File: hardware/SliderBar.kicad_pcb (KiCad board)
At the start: 2 copper layers, 50 x 30.1 mm, 35 parts, among them J1 USB_B_Mini, J2 MOTOR, J3 TAPER_RIGHT, J4 TAPER_LEFT, J5 DEBUG, U1 MIC5205-3.3YM5, U2 MT3608, U3 STM32F072C8Tx, U4 TB6612FNG

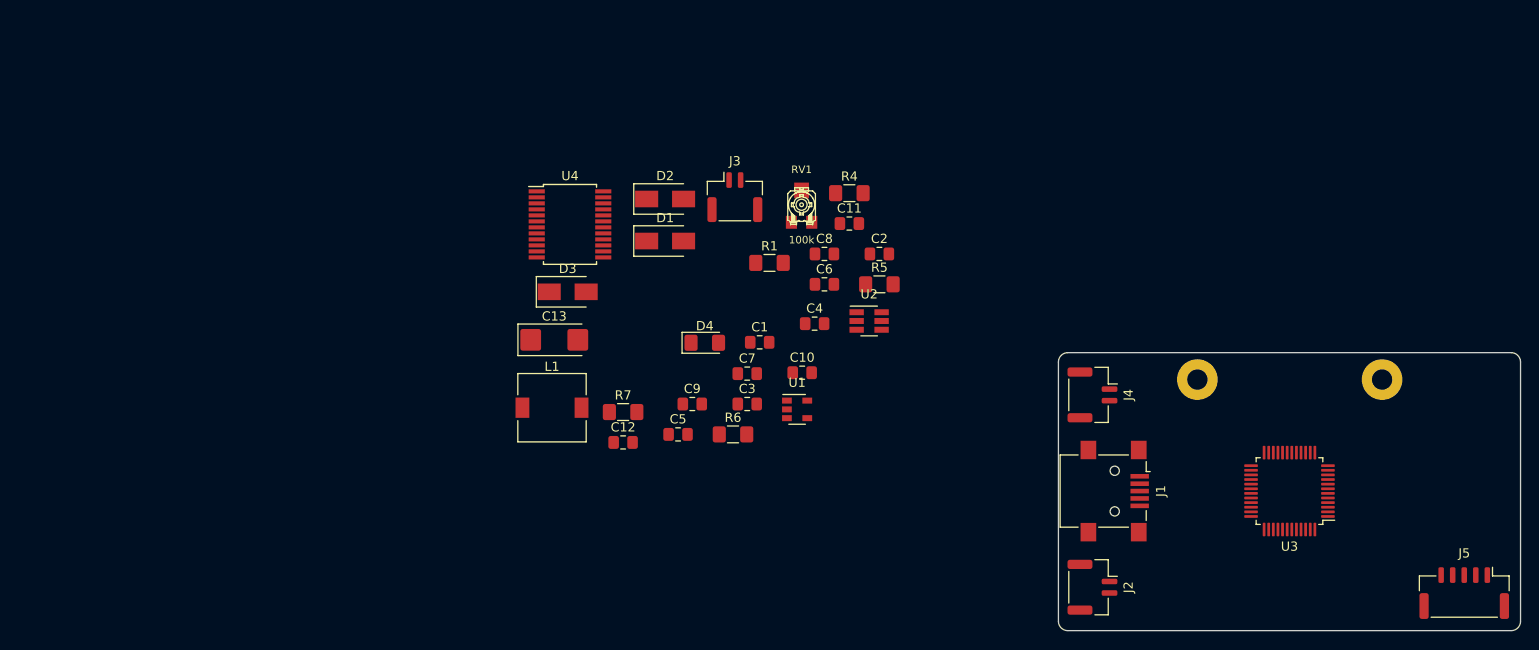
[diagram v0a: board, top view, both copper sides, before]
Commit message: Placed some components, fixed schematic
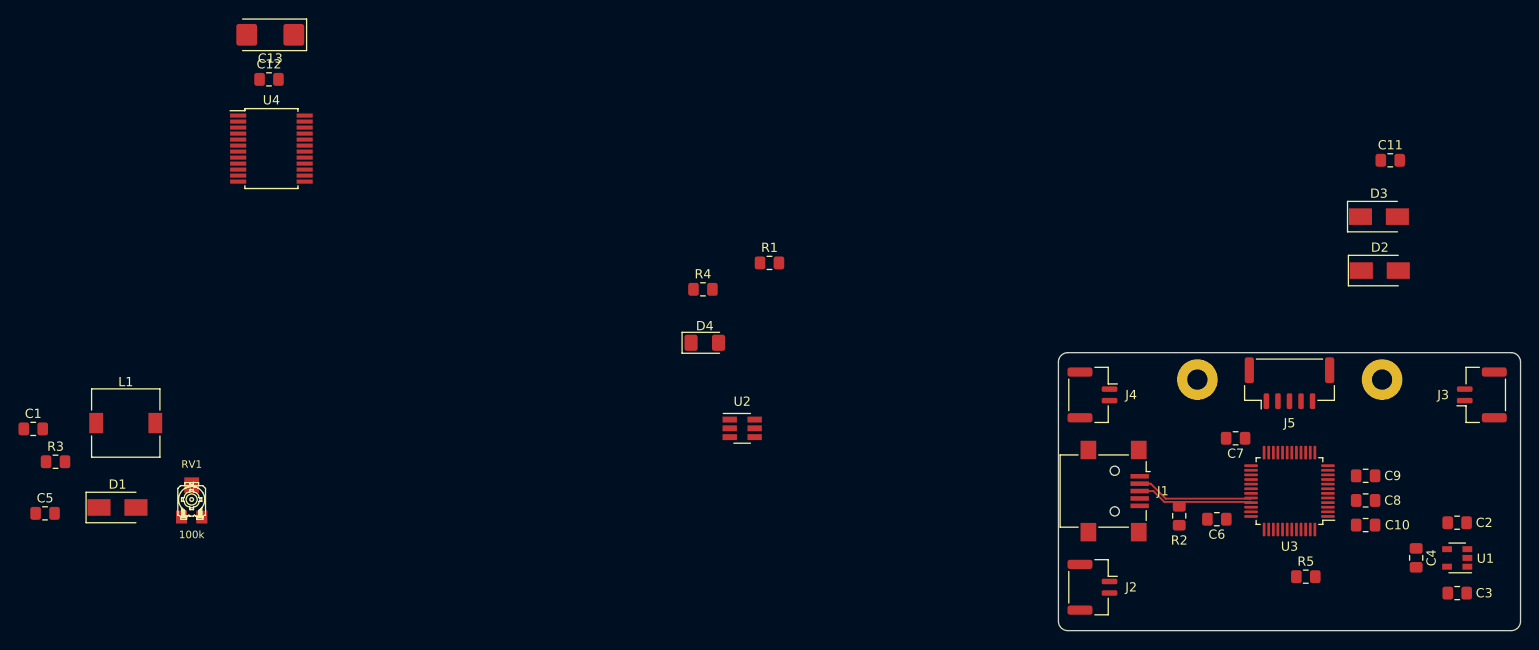
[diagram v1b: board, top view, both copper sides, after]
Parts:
- removed R6: 1k, Resistor_SMD:R_1206_3216Metric_Pad1.42x1.75mm_HandSolder
- removed R7: 10k, Resistor_SMD:R_1206_3216Metric_Pad1.42x1.75mm_HandSolder
- added R2: 1.5k, Resistor_SMD:R_0805_2012Metric_Pad1.15x1.40mm_HandSolder, F.Cu at (150.4, 68.6)
- added R3: 3k, Resistor_SMD:R_0805_2012Metric_Pad1.15x1.40mm_HandSolder, F.Cu at (28.7, 62.7)
- R1: footprint Resistor_SMD:R_1206_3216Metric_Pad1.42x1.75mm_HandSolder -> Resistor_SMD:R_0805_2012Metric_Pad1.15x1.40mm_HandSolder
- R4: value 1.5k -> 1k; footprint Resistor_SMD:R_1206_3216Metric_Pad1.42x1.75mm_HandSolder -> Resistor_SMD:R_0805_2012Metric_Pad1.15x1.40mm_HandSolder
- R5: value 3k -> 10k; footprint Resistor_SMD:R_1206_3216Metric_Pad1.42x1.75mm_HandSolder -> Resistor_SMD:R_0805_2012Metric_Pad1.15x1.40mm_HandSolder
- moved D3 88.2 mm to (172.0, 36.2)
- moved J3 83.7 mm to (183.1, 55.5), turned to 90 degrees
- moved C3 79.6 mm to (180.5, 77.0)
- moved C1 79.2 mm to (26.3, 59.2)
- moved D2 77.8 mm to (172.1, 42.0)
- moved RV1 73.3 mm to (43.4, 66.8)
- moved C9 73.3 mm to (170.6, 64.3)
- moved U1 73.3 mm to (180.5, 73.2), turned to 180 degrees
- moved C4 69.9 mm to (176.0, 73.1), turned to 270 degrees
- moved C5 69.1 mm to (27.6, 68.3)
- moved C2 69.0 mm to (180.5, 69.3), turned to 180 degrees
- moved D1 65.9 mm to (35.4, 67.7)
- moved C8 64.4 mm to (170.6, 66.9)
- moved C10 63.2 mm to (170.6, 69.6)
- moved C11 59.0 mm to (173.2, 30.1)
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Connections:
- R4 pad 1: +3V3 -> +5V
- R4 pad 2: USB_DP -> Net-(D4-Pad2)
- R5 pad 1: GND -> Net-(R5-Pad1)
- R5 pad 2: Net-(R5-Pad2) -> GND
- RV1 pad 2: Net-(R5-Pad2) -> Net-(R3-Pad2)
- U2 pad 3: Net-(R5-Pad2) -> Net-(R3-Pad2)
- U3 pad 44: Net-(R7-Pad1) -> Net-(R5-Pad1)
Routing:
- net USB_DN: track 0.00 -> 12.8 mm
- net USB_DP: track 0.00 -> 12.6 mm
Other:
- net class Default: trace_width 0.1524 -> 0.2032
- net class PowerLowVoltage: trace_width 0.381 -> 0.4064
